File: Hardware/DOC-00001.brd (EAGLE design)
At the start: 22.9 x 16.5 mm, 8 parts

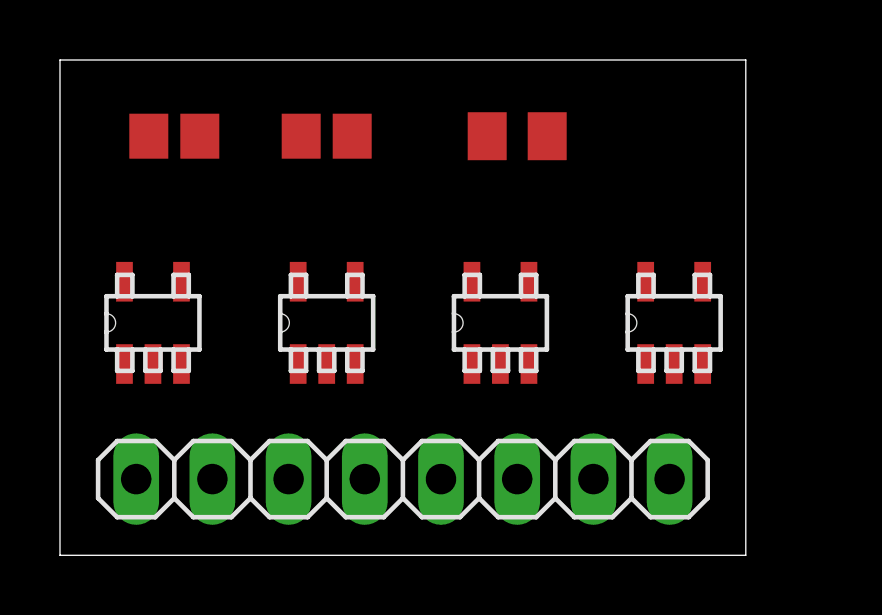
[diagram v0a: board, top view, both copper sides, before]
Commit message: Routed. Needs ground layers.
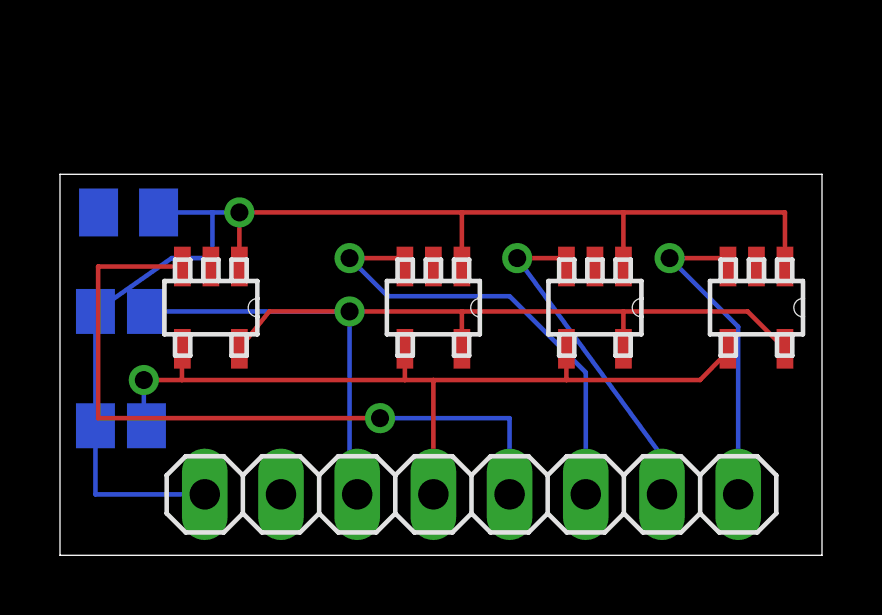
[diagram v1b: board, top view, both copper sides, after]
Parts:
- moved C1 13.2 mm to (2.29, 11.4), flipped to the bottom
- moved R2 11.8 mm to (2.03, 4.32), flipped to the bottom
- moved R1 6.11 mm to (2.03, 8.13), flipped to the bottom
- moved U$2 3.59 mm to (12.4, 8.26), turned to 270 degrees
- moved U$3 3.19 mm to (17.8, 8.26), turned to 270 degrees
- moved U$4 2.79 mm to (23.2, 8.26), turned to 270 degrees
- moved JP1 2.34 mm to (13.7, 2.03)
- moved U$1 2.00 mm to (5.03, 8.26), turned to 270 degrees
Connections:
- net AIN0: now also JP1.5; no longer JP1.3
- net AIN1: now also JP1.6; no longer JP1.4
- net AIN2: now also JP1.7; no longer JP1.5
- net AIN3: now also JP1.8; no longer JP1.6
- net SCL: now also JP1.3; no longer JP1.7
- net SDA: now also JP1.4; no longer JP1.8
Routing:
- net VDD: track 0.00 -> 43.8 mm, vias 0 -> 1
- net SCL: track 0.00 -> 34.8 mm, vias 0 -> 1
- net SDA: track 0.00 -> 28.6 mm, vias 0 -> 1
- net AIN0: track 0.00 -> 24.1 mm, vias 0 -> 1
- net AIN1: track 0.00 -> 15.5 mm, vias 0 -> 1
- net AIN2: track 0.00 -> 11.2 mm, vias 0 -> 1
- net AIN3: track 0.00 -> 10.9 mm, vias 0 -> 1
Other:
- board size 22.9 x 16.5 mm -> 25.4 x 12.7 mm
